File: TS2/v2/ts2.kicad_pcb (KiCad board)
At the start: 2 copper layers, 104 parts, among them P1 FTDI (TERMINAL), P2 FTDI (HOST), P3 +5V POWER, SW1 RESET, SW2 SINGLE STEP/RUN, SW3 STEP, SW4 ABORT, SW5 POWER, U1 555, U10 74LS32, U11 HM6264, U12 28C64, U13 HM6264, U14 28C64, U15 HM6264, U16 28C64, U17 HM6264, U18 28C64, U19 74LS20, U2 8 MHz, U20 74LS74, U21 74LS161, U22 74LS161, U23 74LS74, U24 74LS260, U25 74LS260, U26 74LS138, U27 25LS2548, U28 74LS148, U29 6850, U3 74LS00, U30 6850, U31 MC14411, U32 74LS138, U33 74LS138, U34 74LS00, U35 74LS74, U4 74LS06, U5 74LS04, U6 68000, U7 74LS08, U8 74LS32, U9 74LS32, Y1 1.842MHz

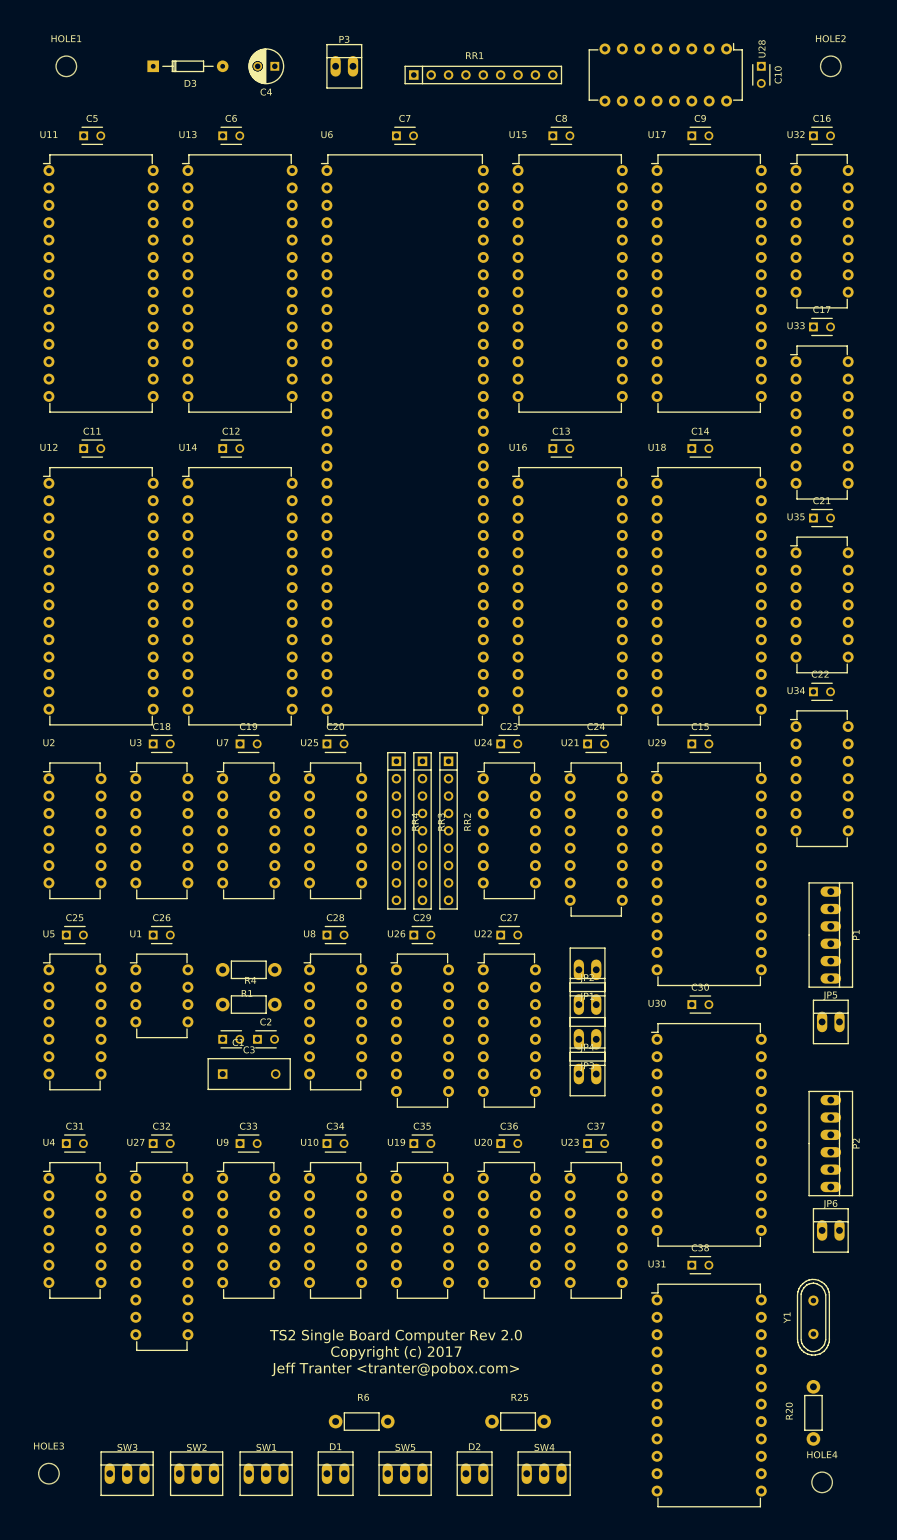
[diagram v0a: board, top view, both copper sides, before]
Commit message: Working on PCB layout.
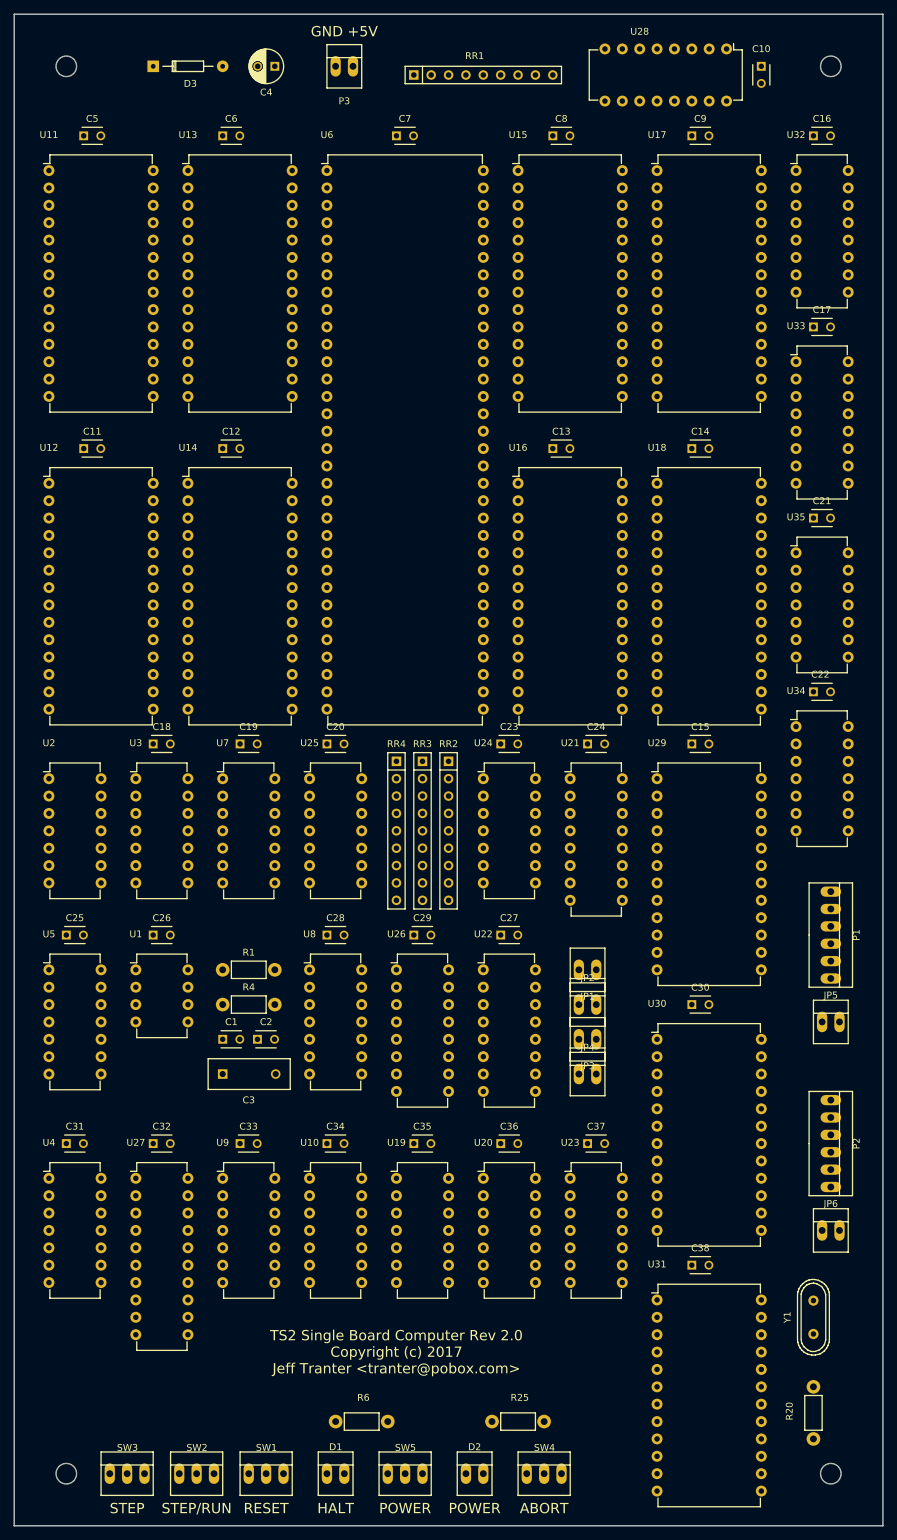
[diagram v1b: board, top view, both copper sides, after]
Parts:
- moved HOLE3 2.54 mm to (30.5, 228.6)
- moved HOLE4 1.80 mm to (142.2, 228.6)
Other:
- board outline added: 127 x 221 mm
- board text added: "ABORT"
- board text added: "GND +5V"
- board text added: "HALT"
- board text added: "POWER"
- board text added: "RESET"
- board text added: "STEP"
- board text added: "STEP/RUN"
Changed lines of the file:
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@@
     (links 625)
     (no_connects 625)
-    (area 21.451474 16.783095 150.730046 235.84626)
+    (area 22.784999 15.164999 150.730046 236.295001)
     (thickness 1.6)
-    (drawings 1)
+    (drawings 13)
     (tracks 0)
     (zones 0)
@@
     (descr "Capacitor 3mm Disc, Pitch 2.5mm")
     (tags Capacitor)
-    (fp_text reference C1 (at 2.286 0.508) (layer F.SilkS)
+    (fp_text reference C1 (at 1.27 -2.54) (layer F.SilkS)
       (effects (font (size 1 1) (thickness 0.15)))
     )
@@
     (descr "Capacitor 3mm Disc, Pitch 2.5mm")
     (tags Capacitor)
-    (fp_text reference C2 (at 1.25 -2.5) (layer F.SilkS)
+    (fp_text reference C2 (at 1.27 -2.54) (layer F.SilkS)
       (effects (font (size 1 1) (thickness 0.15)))
     )
@@
     (descr "Capacitor 12mm Disc, Pitch 7.75mm")
     (tags Capacitor)
-    (fp_text reference C3 (at 3.875 -3.5) (layer F.SilkS)
+    (fp_text reference C3 (at 3.81 3.81) (layer F.SilkS)
       (effects (font (size 1 1) (thickness 0.15)))
     )
@@
     (descr "Capacitor 3mm Disc, Pitch 2.5mm")
     (tags Capacitor)
-    (fp_text reference C10 (at 1.25 -2.5 270) (layer F.SilkS)
+    (fp_text reference C10 (at -2.54 0 360) (layer F.SilkS)
       (effects (font (size 1 1) (thickness 0.15)))
     )
-    (fp_text value 0.1uF (at 6.096 0 270) (layer F.Fab)
+    (fp_text value 0.1uF (at 5.08 0 360) (layer F.Fab)
       (effects (font (size 1 1) (thickness 0.15)))
     )
@@
     (at 71.12 22.86)
     (attr virtual)
-    (fp_text reference P3 (at 0 -3.9) (layer F.SilkS)
+    (fp_text reference P3 (at 0 5.08) (layer F.SilkS)
       (effects (font (size 1 1) (thickness 0.15)))
     )
@@
     (descr "Resistor, Axial,  RM 7.62mm, 1/3W,")
     (tags "Resistor Axial RM 7.62mm 1/3W R3")
-    (fp_text reference R1 (at 4.05892 -3.50012 180) (layer F.SilkS)
+    (fp_text reference R1 (at 3.81 2.54 180) (layer F.SilkS)
       (effects (font (size 1 1) (thickness 0.15)))
     )
@@
     (descr "Resistor, Axial,  RM 7.62mm, 1/3W,")
     (tags "Resistor Axial RM 7.62mm 1/3W R3")
-    (fp_text reference R4 (at 4.05892 -3.50012) (layer F.SilkS)
+    (fp_text reference R4 (at 3.81 -2.54) (layer F.SilkS)
       (effects (font (size 1 1) (thickness 0.15)))
     )
@@
       (effects (font (size 1 1) (thickness 0.15)))
     )
-    (fp_text value 4.7K (at 0 2.032) (layer F.Fab)
+    (fp_text value 4.7K (at 0 3.81) (layer F.Fab)
       (effects (font (size 1 1) (thickness 0.15)))
     )
@@
     (descr "8 R pack")
     (tags R)
-    (fp_text reference RR2 (at -1.27 -2.794 270) (layer F.SilkS)
+    (fp_text reference RR2 (at -12.7 0 360) (layer F.SilkS)
       (effects (font (size 1 1) (thickness 0.15)))
     )
@@
     (descr "8 R pack")
     (tags R)
-    (fp_text reference RR3 (at -1.27 -2.794 270) (layer F.SilkS)
+    (fp_text reference RR3 (at -12.7 0 360) (layer F.SilkS)
       (effects (font (size 1 1) (thickness 0.15)))
     )
@@
     (descr "8 R pack")
     (tags R)
-    (fp_text reference RR4 (at -1.27 -2.794 270) (layer F.SilkS)
+    (fp_text reference RR4 (at -12.7 0 360) (layer F.SilkS)
       (effects (font (size 1 1) (thickness 0.15)))
     )
@@
     (descr "16-lead dip package, row spacing 7.62 mm (300 mils)")
     (tags "dil dip 2.54 300")
-    (fp_text reference U28 (at 0 -5.22 270) (layer F.SilkS)
+    (fp_text reference U28 (at -2.54 12.7 360) (layer F.SilkS)
       (effects (font (size 1 1) (thickness 0.15)))
     )
-    (fp_text value 74LS148 (at 0 -3.72 270) (layer F.Fab)
+    (fp_text value 74LS148 (at -2.54 7.62 360) (layer F.Fab)
       (effects (font (size 1 1) (thickness 0.15)))
     )
@@
     (descr "Mounting hole, Befestigungsbohrung, 3mm, No Annular, Kein Restring,")
     (tags "Mounting hole, Befestigungsbohrung, 3mm, No Annular, Kein Restring,")
-    (fp_text reference HOLE1 (at 0 -4.0005) (layer F.SilkS)
+    (fp_text reference HOLE1 (at 0 -4.0005) (layer F.SilkS) hide
       (effects (font (size 1 1) (thickness 0.15)))
     )
@@
     (descr "Mounting hole, Befestigungsbohrung, 3mm, No Annular, Kein Restring,")
     (tags "Mounting hole, Befestigungsbohrung, 3mm, No Annular, Kein Restring,")
-    (fp_text reference HOLE2 (at 0 -4.0005) (layer F.SilkS)
+    (fp_text reference HOLE2 (at 0 -4.0005) (layer F.SilkS) hide
       (effects (font (size 1 1) (thickness 0.15)))
     )
@@
   )
   (module Mounting_Holes:MountingHole_3mm (layer F.Cu)
-    (at 140.97 229.87)
+    (at 142.24 228.6)
     (descr "Mounting hole, Befestigungsbohrung, 3mm, No Annular, Kein Restring,")
     (tags "Mounting hole, Befestigungsbohrung, 3mm, No Annular, Kein Restring,")
-    (fp_text reference HOLE4 (at 0 -4.0005) (layer F.SilkS)
+    (fp_text reference HOLE4 (at 0 -4.0005) (layer F.SilkS) hide
       (effects (font (size 1 1) (thickness 0.15)))
     )
@@
   )
   (module Mounting_Holes:MountingHole_3mm (layer F.Cu)
-    (at 27.94 228.6)
+    (at 30.48 228.6)
     (descr "Mounting hole, Befestigungsbohrung, 3mm, No Annular, Kein Restring,")
     (tags "Mounting hole, Befestigungsbohrung, 3mm, No Annular, Kein Restring,")
-    (fp_text reference HOLE3 (at 0 -4.0005) (layer F.SilkS)
+    (fp_text reference HOLE3 (at 0 -4.0005) (layer F.SilkS) hide
       (effects (font (size 1 1) (thickness 0.15)))
     )
@@
     (pad 1 thru_hole circle (at 0 0) (size 3 3) (drill 3) (layers))
   )
+  (gr_text POWER (at 80.01 233.68) (layer F.SilkS)
+    (effects (font (size 1.5 1.5) (thickness 0.3)))
+  )
+  (gr_text POWER (at 90.17 233.68) (layer F.SilkS)
+    (effects (font (size 1.5 1.5) (thickness 0.3)))
+  )
+  (gr_text ABORT (at 100.33 233.68) (layer F.SilkS)
+    (effects (font (size 1.5 1.5) (thickness 0.3)))
+  )
+  (gr_text HALT (at 69.85 233.68) (layer F.SilkS)
+    (effects (font (size 1.5 1.5) (thickness 0.3)))
+  )
+  (gr_text RESET (at 59.69 233.68) (layer F.SilkS)
+    (effects (font (size 1.5 1.5) (thickness 0.3)))
+  )
+  (gr_text STEP/RUN (at 49.53 233.68) (layer F.SilkS)
+    (effects (font (size 1.5 1.5) (thickness 0.3)))
+  )
+  (gr_text STEP (at 39.37 233.68) (layer F.SilkS)
+    (effects (font (size 1.5 1.5) (thickness 0.3)))
+  )
+  (gr_text "GND +5V" (at 71.12 17.78) (layer F.SilkS)
+    (effects (font (size 1.5 1.5) (thickness 0.3)))
+  )
+  (gr_line (start 22.86 236.22) (end 22.86 15.24) (angle 90) (layer Edge.Cuts) (width 0.15))
+  (gr_line (start 149.86 236.22) (end 22.86 236.22) (angle 90) (layer Edge.Cuts) (width 0.15))
+  (gr_line (start 149.86 15.24) (end 149.86 236.22) (angle 90) (layer Edge.Cuts) (width 0.15))
+  (gr_line (start 22.86 15.24) (end 149.86 15.24) (angle 90) (layer Edge.Cuts) (width 0.15))
   (gr_text "TS2 Single Board Computer Rev 2.0\nCopyright (c) 2017\nJeff Tranter <tranter@pobox.com>" (at 78.74 210.82) (layer F.SilkS)
     (effects (font (size 1.5 1.5) (thickness 0.3)))

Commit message: Initial PCB routing.
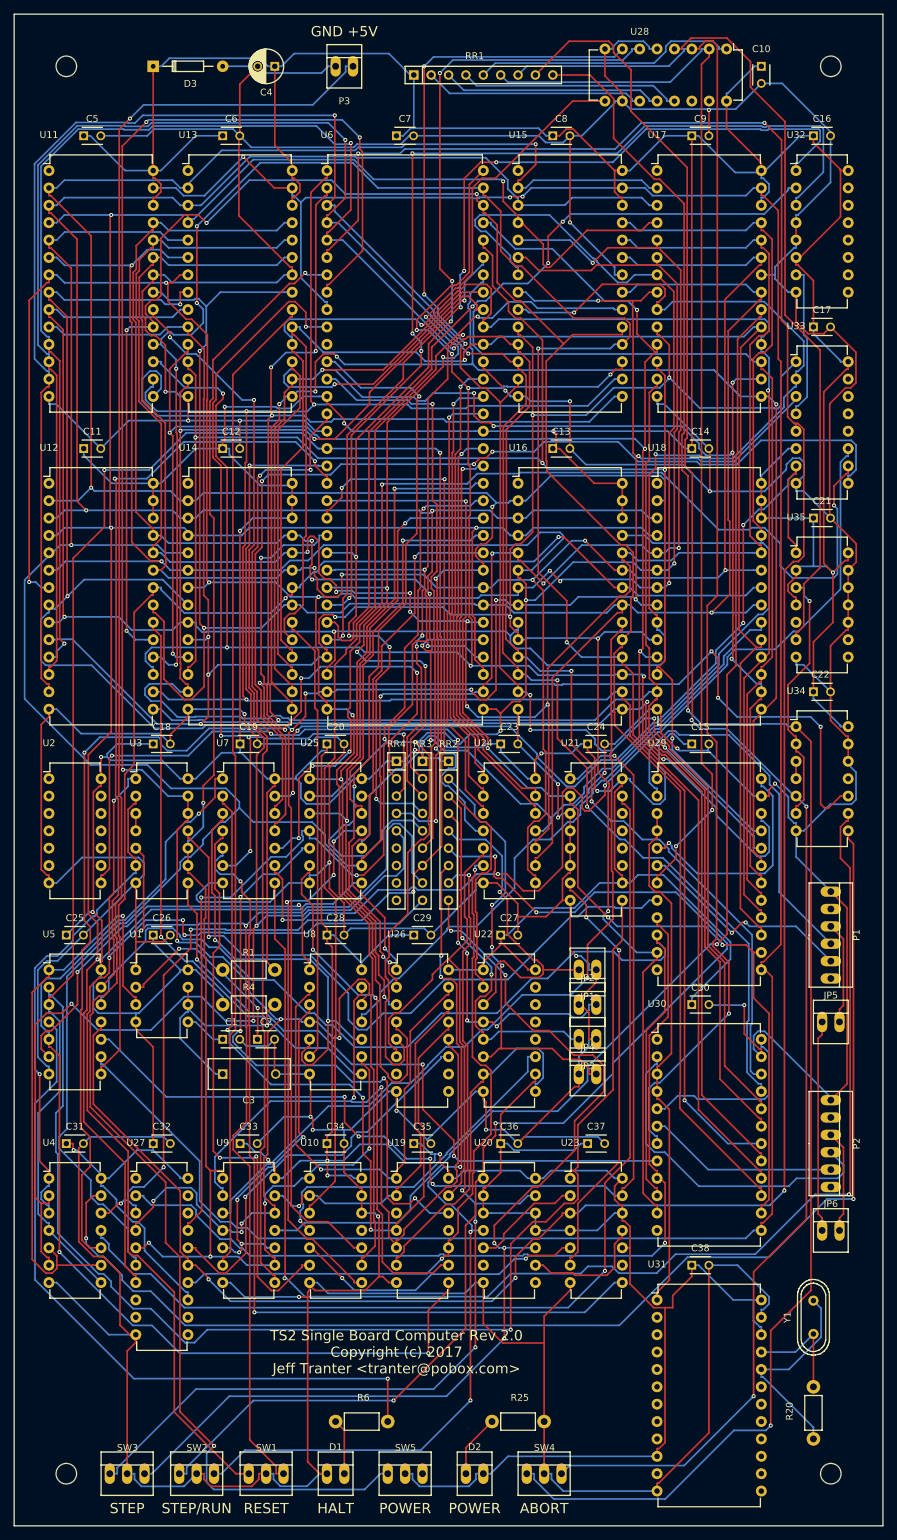
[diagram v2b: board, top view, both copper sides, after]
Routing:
- net GND: track 0.00 -> 1448.8 mm, vias 0 -> 23
- net VCC: track 0.00 -> 1344.8 mm, vias 0 -> 15
- net A07: track 0.00 -> 427.9 mm, vias 0 -> 5
- net A06: track 0.00 -> 421.2 mm, vias 0 -> 6
- net A03: track 0.00 -> 391.6 mm, vias 0 -> 9
- net A04: track 0.00 -> 389.1 mm, vias 0 -> 8
- net A08: track 0.00 -> 387.0 mm, vias 0 -> 5
- net A01: track 0.00 -> 384.7 mm, vias 0 -> 9
- net R/W*: track 0.00 -> 383.7 mm, vias 0 -> 3
- net AS*: track 0.00 -> 380.3 mm, vias 0 -> 5
- net A09: track 0.00 -> 324.5 mm, vias 0 -> 5
- net D02: track 0.00 -> 322.1 mm, vias 0 -> 5
- net D05: track 0.00 -> 313.9 mm, vias 0 -> 8
- net A13: track 0.00 -> 313.3 mm, vias 0 -> 5
- net D03: track 0.00 -> 312.5 mm, vias 0 -> 5
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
